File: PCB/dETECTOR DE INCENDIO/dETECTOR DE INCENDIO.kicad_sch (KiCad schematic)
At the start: 4 parts, among them J1 Screw_Terminal_01x02, J2 Conn_01x03, J3 Conn_01x03, J4 DHT11

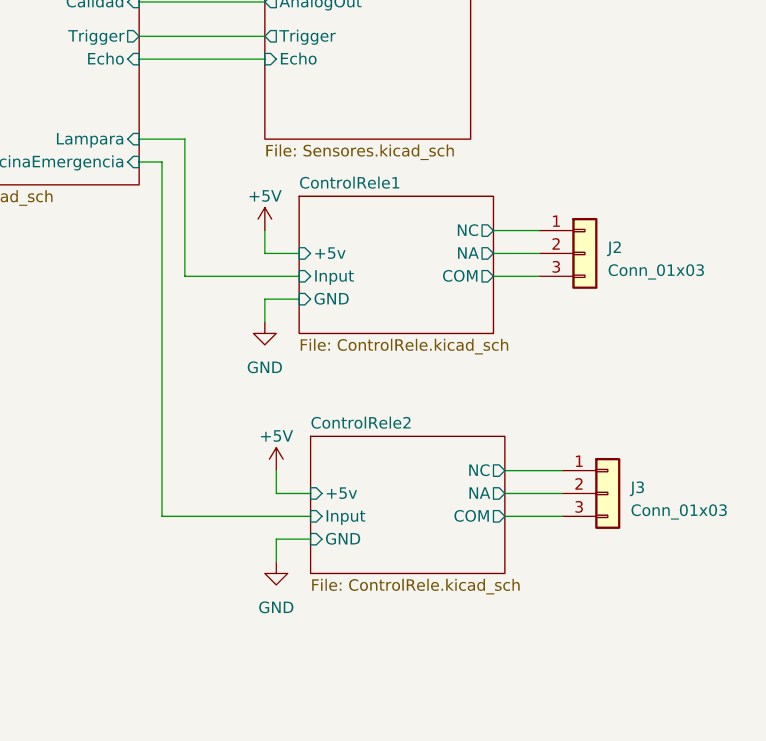
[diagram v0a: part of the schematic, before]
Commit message: Se crea dise;o preliminar de PCB
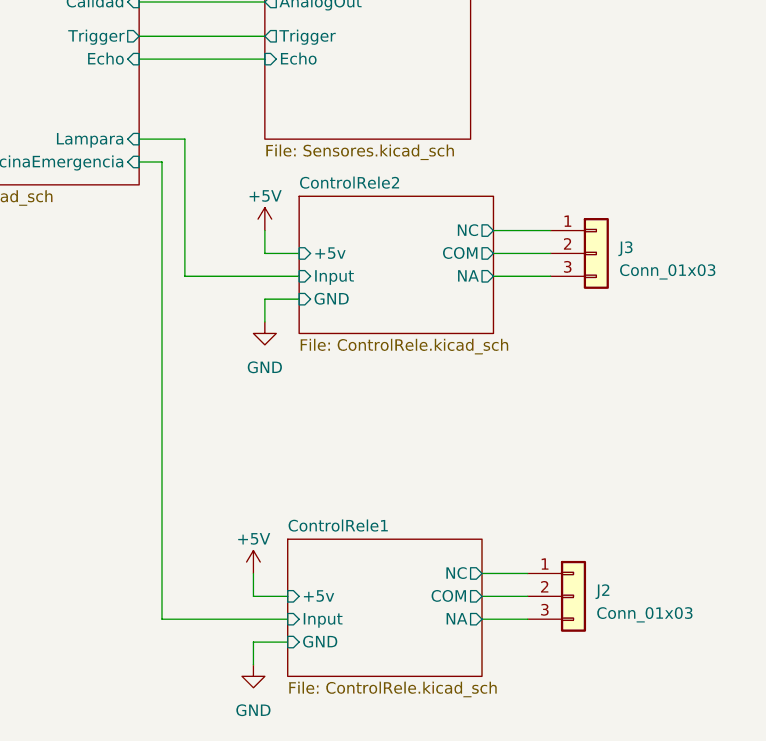
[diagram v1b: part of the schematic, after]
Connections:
- net ControlRele1/COM: now also J2.2 (Pin_2); no longer J2.3 (Pin_3)
- net ControlRele1/NA: now also J2.3 (Pin_3); no longer J2.2 (Pin_2)
- net ControlRele2/COM: now also J3.2 (Pin_2); no longer J3.3 (Pin_3)
- net ControlRele2/NA: now also J3.3 (Pin_3); no longer J3.2 (Pin_2)
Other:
- moved on the sheet: J2, J3
